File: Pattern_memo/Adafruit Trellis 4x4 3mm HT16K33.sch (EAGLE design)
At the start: 41 parts, among them U1 HT16K33 28SOP

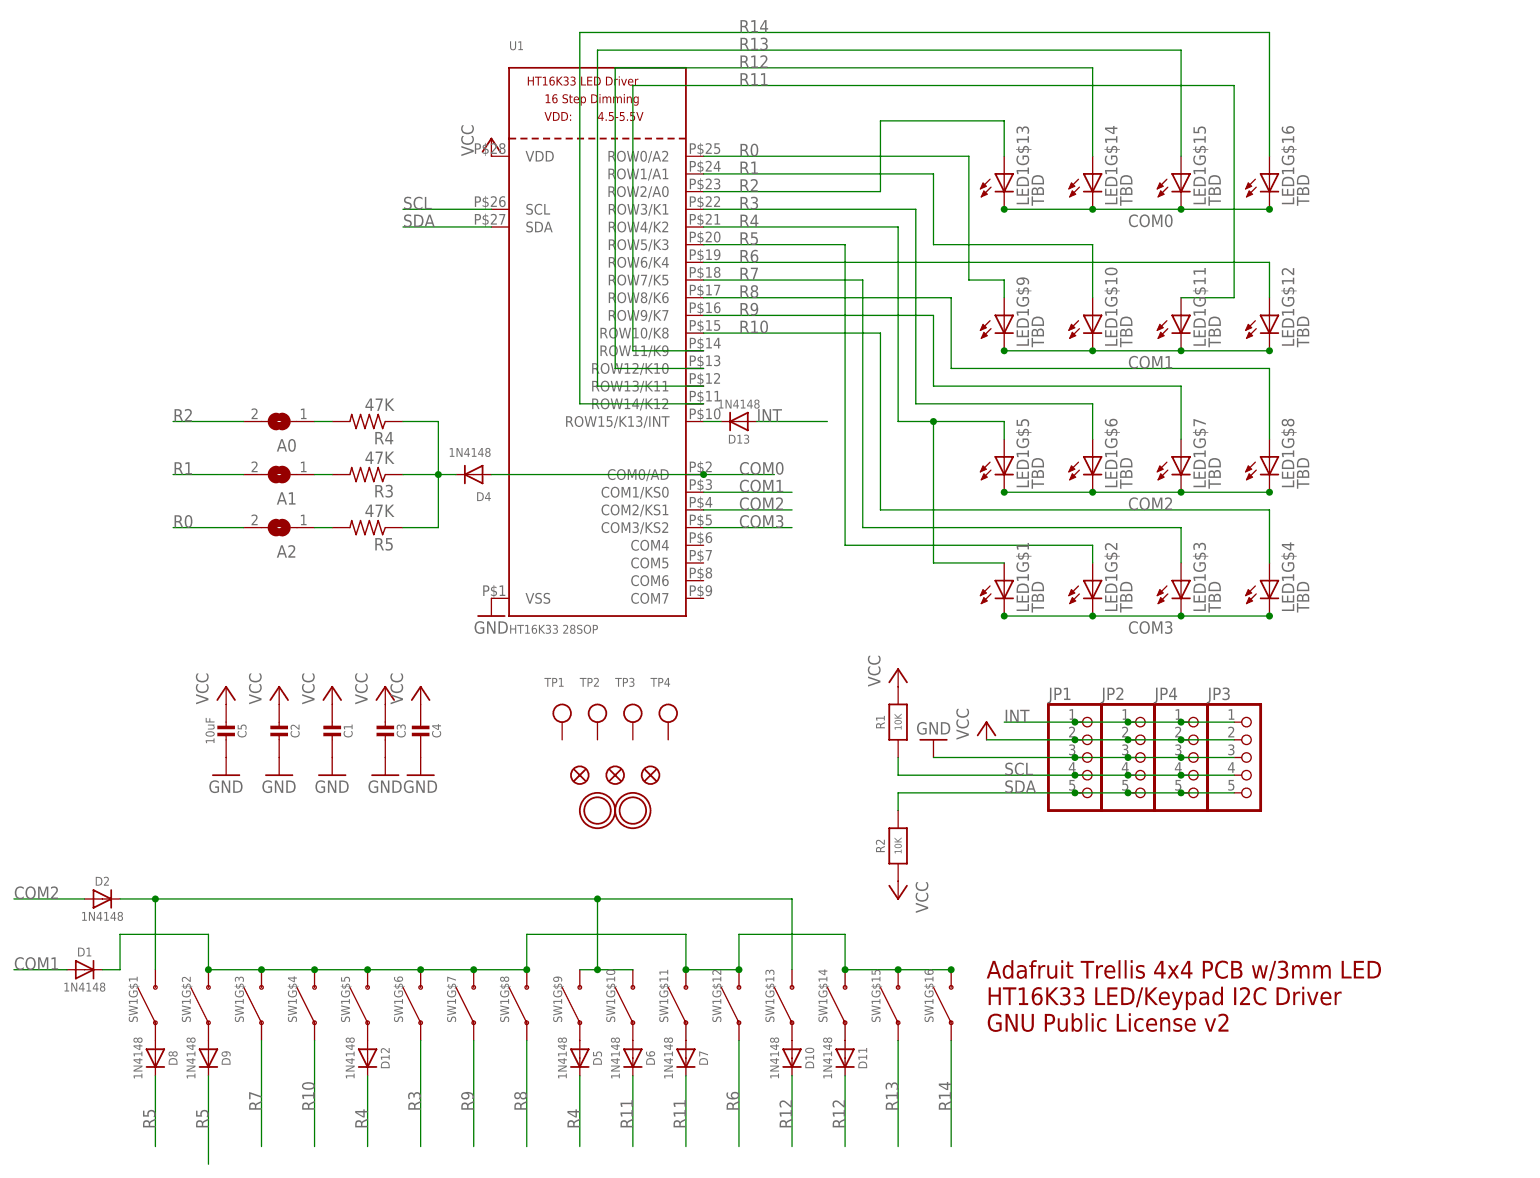
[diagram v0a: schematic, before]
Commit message: updated pcb board
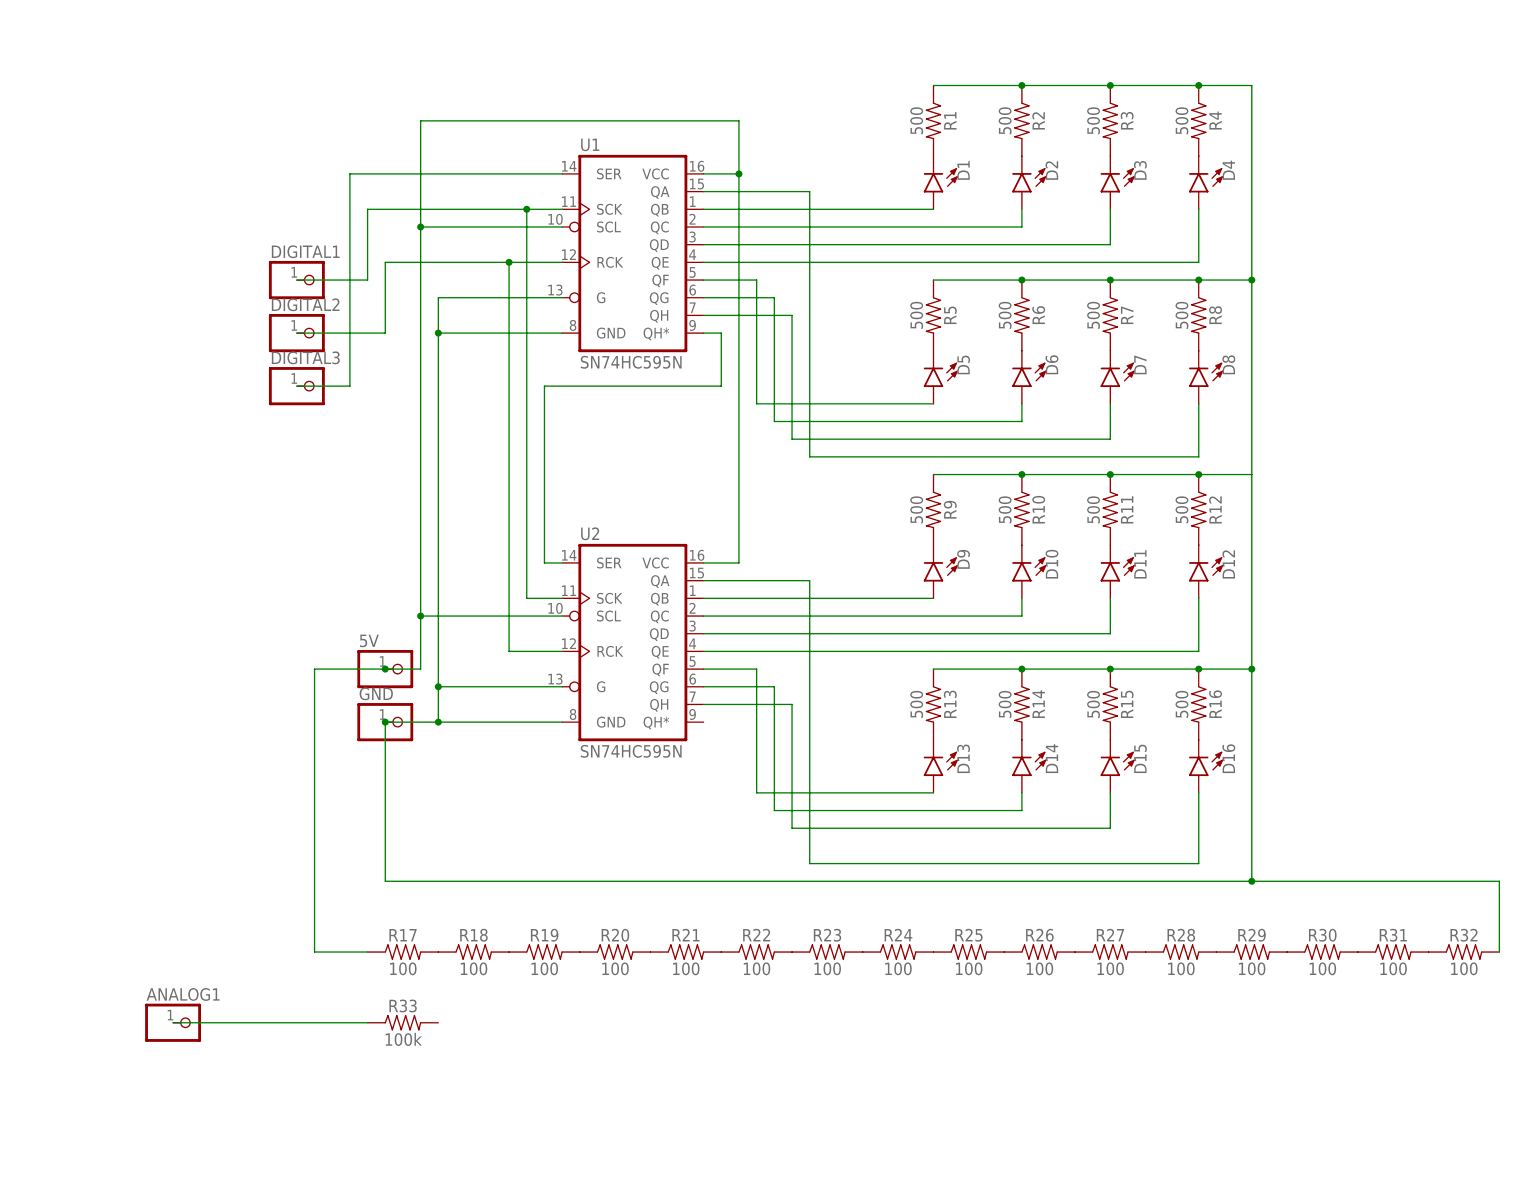
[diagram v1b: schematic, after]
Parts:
- removed A0, A1, A2: (no value), microbuilder:SOLDERJUMPERREFLOW_NOPASTE
- removed C1, C2, C3, C4: (no value), microbuilder:CAP_CERAMIC_0805
- removed C5: 10uF, microbuilder:CAP_CERAMIC_0805
- removed FID1, FID2, FID3: FIDUCIAL"", microbuilder:FIDUCIAL""
- removed JP1, JP2, JP3, JP4: (no value), microbuilder:HEADER-1X5EDGESMT
- removed LED1: TBD, microbuilder:LED-3MM-4X4GRID-3MM
- removed SW1: (no value), microbuilder:SWITCH-SILICON-4X4GRID-10MM-5.4MM
- removed TP1, TP2, TP3, TP4: (no value), microbuilder:TESTPOINT
- removed U$1, U$2: MOUNTINGHOLE2.5, microbuilder:MOUNTINGHOLE2.5
- added 5V, ANALOG1, DIGITAL1, DIGITAL2, DIGITAL3, GND: (no value), adafruit:PINHD-1X1
- added D14, D15, D16, D3: (no value), SparkFun-LED:LED3MM
- added R10, R11, R12, R13, R14, R15, R16, R6, R7, R8, R9: 500, SparkFun-Resistors:RESISTOR0603
- added R17, R18, R19, R20, R21, R22, R23, R24, R25, R26, R27, R28, R29, R30, R31, R32: 100, SparkFun-Resistors:100OHM-0603-1/10W-1%
- added R33: 100k, SparkFun-Resistors:100KOHM-0603-1/10W-1%
- added U2: SN74HC595N, SparkFun-IC-Logic:74HC595N
- D1, D10, D11, D12, D13, D2, D5, D6, D7, D8, D9: value 1N4148 -> (none); device microbuilder:DIODESOD-323 -> SparkFun-LED:LED3MM
- D4: value 1N4148 -> (none); device adafruit:DIODESOD-323F -> SparkFun-LED:LED3MM
- R1, R2: value 10K -> 500; device microbuilder:RESISTOR_0805 -> SparkFun-Resistors:RESISTOR0603
- R3, R4, R5: value 47K -> 500; device rcl:R-US_R0805 -> SparkFun-Resistors:RESISTOR0603
- U1: value HT16K33 28SOP -> SN74HC595N; device microbuilder:HT16K33_SOP28 -> SparkFun-IC-Logic:74HC595N
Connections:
- removed net COM0: D4.A, LED1G$13.C, LED1G$14.C, LED1G$15.C, LED1G$16.C, U1.COM0/AD
- removed net COM1: D1.A, LED1G$10.C, LED1G$11.C, LED1G$12.C, LED1G$9.C, U1.COM1/KS0
- removed net COM2: D2.A, LED1G$5.C, LED1G$6.C, LED1G$7.C, LED1G$8.C, U1.COM2/KS1
- removed net COM3: LED1G$1.C, LED1G$2.C, LED1G$3.C, LED1G$4.C, U1.COM3/KS2
- removed net GND: C1.1, C2.1, C3.1, C4.1, C5.1, JP1.3, JP2.3, JP3.3, JP4.3, U1.VSS
- removed net INT: D13.A, JP1.1, JP2.1, JP3.1, JP4.1
- removed net R0: A2.2, LED1G$9.A, U1.ROW0/A2
- removed net R1: A1.2, LED1G$10.A, U1.ROW1/A1
- removed net R10: LED1G$4.A, SW1G$4.P$1, U1.ROW10/K8
- removed net R11: D6.C, D7.C, LED1G$11.A, U1.ROW11/K9
- removed net R12: D10.C, D11.C, LED1G$14.A, U1.ROW12/K10
- removed net R13: LED1G$15.A, SW1G$15.P$1, U1.ROW13/K11
- removed net R14: LED1G$16.A, SW1G$16.P$1, U1.ROW14/K12
- removed net R2: A0.2, LED1G$13.A, U1.ROW2/A0
- removed net R3: LED1G$6.A, SW1G$6.P$1, U1.ROW3/K1
- removed net R4: D12.C, D5.C, LED1G$1.A, LED1G$5.A, U1.ROW4/K2
- removed net R5: D8.C, D9.C, LED1G$2.A, U1.ROW5/K3
- removed net R6: LED1G$12.A, SW1G$12.P$1, U1.ROW6/K4
- removed net R7: LED1G$3.A, SW1G$3.P$1, U1.ROW7/K5
- removed net R8: LED1G$8.A, SW1G$8.P$1, U1.ROW8/K6
- removed net R9: LED1G$7.A, SW1G$7.P$1, U1.ROW9/K7
- removed net SCL: JP1.4, JP2.4, JP3.4, JP4.4, R1.1, U1.SCL
- removed net SDA: JP1.5, JP2.5, JP3.5, JP4.5, R2.2, U1.SDA
- removed net VCC: C1.2, C2.2, C3.2, C4.2, C5.2, JP1.2, JP2.2, JP3.2, JP4.2, R1.2, R2.1, U1.VDD
- new net N$13: D7.C, R7.2
- new net N$14: GND.1, R1.1, R10.1, R11.1, R12.1, R13.1, R14.1, R15.1, R16.1, R2.1, R3.1, R32.2, R4.1, R5.1, R6.1, R7.1, R8.1, R9.1, U1.G, U1.GND, U2.G, U2.GND
- new net N$15: D8.C, R8.2
- new net N$17: D10.C, R10.2
- new net N$18: D11.C, R11.2
- new net N$21: D14.C, R14.2
- new net N$22: D15.C, R15.2
- new net N$23: D16.C, R16.2
- new net N$24: D1.A, U1.QB
- new net N$25: D2.A, U1.QC
- new net N$26: D3.A, U1.QD
- new net N$27: D4.A, U1.QE
- new net N$28: D5.A, U1.QF
- new net N$29: D6.A, U1.QG
- new net N$30: D7.A, U1.QH
- new net N$31: D8.A, U1.QA
- new net N$32: D9.A, U2.QB
- new net N$33: D10.A, U2.QC
- new net N$34: D11.A, U2.QD
- new net N$35: 5V.1, R17.1, U1.SCL, U1.VCC, U2.SCL, U2.VCC
- new net N$36: D12.A, U2.QE
- new net N$37: R18.2, R19.1
- new net N$38: D13.A, U2.QF
- new net N$39: D14.A, U2.QG
- new net N$40: R19.2, R20.1
- new net N$41: D15.A, U2.QH
- new net N$42: R20.2, R21.1
- new net N$43: R21.2, R22.1
- new net N$44: R22.2, R23.1
- new net N$45: R23.2, R24.1
- new net N$46: R24.2, R25.1
- new net N$47: R25.2, R26.1
- new net N$48: R26.2, R27.1
- new net N$49: R27.2, R28.1
- new net N$50: R28.2, R29.1
- new net N$51: R29.2, R30.1
- new net N$52: R30.2, R31.1
- new net N$53: R31.2, R32.1
- new net N$54: D16.A, U2.QA
- net N$1: now also R17.2, R18.1; no longer D2.C, SW1G$1.P$2, SW1G$10.P$2, SW1G$13.P$2, SW1G$9.P$2
- net N$10: now also D4.C, R4.2; no longer D10.A, SW1G$13.P$1
- net N$11: now also D5.C, R5.2; no longer D11.A, SW1G$14.P$1
- net N$12: now also D6.C, R6.2; no longer D12.A, SW1G$5.P$1
- net N$16: now also D9.C, R9.2; no longer D4.C, R3.1, R4.1, R5.1
- net N$19: now also D12.C, R12.2; no longer A1.1, R3.2
- net N$2: now also ANALOG1.1, R33.1; no longer D13.C, U1.ROW15/K13/INT
- net N$20: now also D13.C, R13.2; no longer A0.1, R4.2
- net N$3: now also DIGITAL3.1, U1.SER; no longer D5.A, SW1G$9.P$1
- net N$4: now also DIGITAL1.1, U1.SCK, U2.SCK; no longer D6.A, SW1G$10.P$1
- net N$5: now also DIGITAL2.1, U1.RCK, U2.RCK; no longer D1.C, SW1G$11.P$2, SW1G$12.P$2, SW1G$14.P$2, SW1G$15.P$2, SW1G$16.P$2, SW1G$2.P$2, SW1G$3.P$2, SW1G$4.P$2, SW1G$5.P$2, SW1G$6.P$2, SW1G$7.P$2, SW1G$8.P$2
- net N$6: now also D1.C, R1.2; no longer D7.A, SW1G$11.P$1
- net N$7: now also D2.C, R2.2; no longer D8.A, SW1G$1.P$1
- net N$8: now also U1.QH*, U2.SER; no longer D9.A, SW1G$2.P$1
- net N$9: now also D3.C, R3.2; no longer A2.1, R5.2
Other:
- note removed: "Adafruit Trellis 4x4 PCB w/3mm LED HT16K33 LED/Keypad I2C Driver GNU Public License v2"
- moved on the sheet: R3, R4, R5

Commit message: schematic & board finished
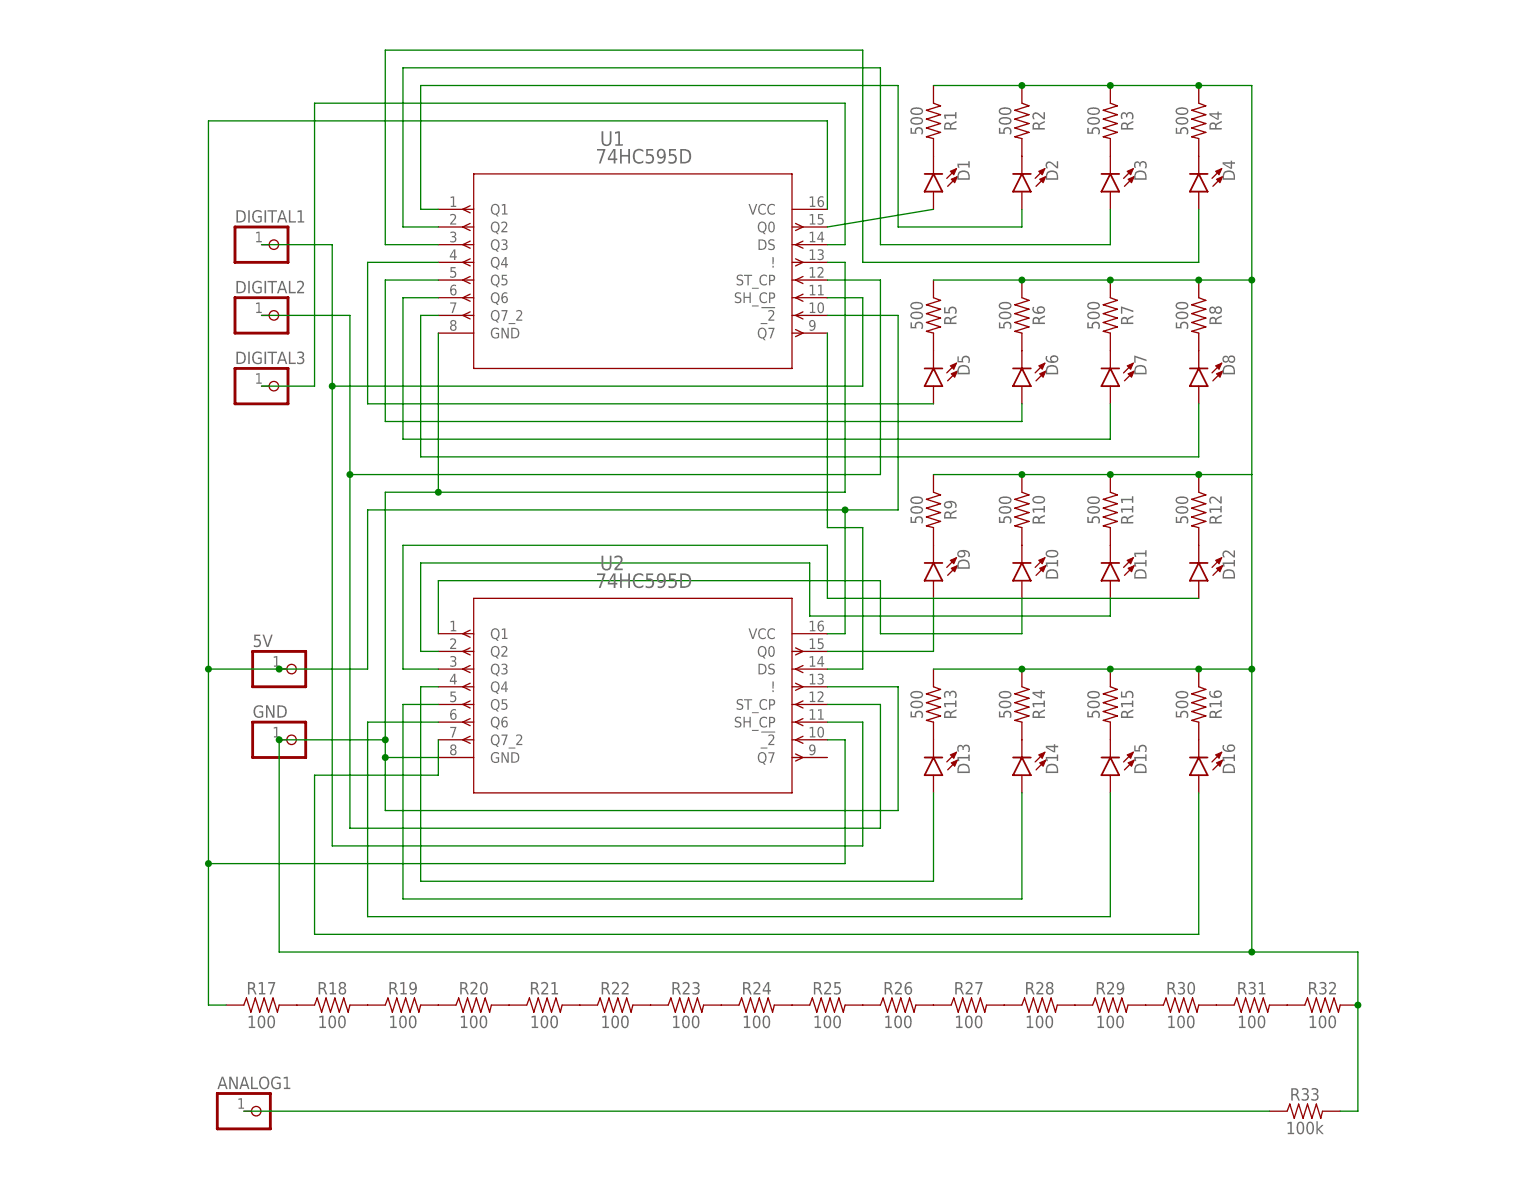
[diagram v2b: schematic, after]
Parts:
- U1, U2: value SN74HC595N -> 74HC595D; device SparkFun-IC-Logic:74HC595N -> Shift_Register:74HC595D
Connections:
- removed net N$34: D11.A, U2.QD
- new net N$55: DIGITAL1.1, U1.SH_CP, U2.SH_CP
- net N$14: now also D1.A, U1.Q0; no longer GND.1, R1.1, R10.1, R11.1, R12.1, R13.1, R14.1, R15.1, R16.1, R2.1, R3.1, R32.2, R4.1, R5.1, R6.1, R7.1, R8.1, R9.1, U1.G, U1.GND, U2.G, U2.GND
- net N$24: now also D5.A, U1.Q4; no longer D1.A, U1.QB
- net N$25: now also U1.Q1; no longer U1.QC
- net N$26: now also U1.Q2; no longer U1.QD
- net N$27: now also U1.Q3; no longer U1.QE
- net N$28: now also U1.Q7, U2.DS; no longer D5.A, U1.QF
- net N$29: now also U1.Q5; no longer U1.QG
- net N$3: now also U1.DS; no longer U1.SER
- net N$30: now also U1.Q6; no longer U1.QH
- net N$31: now also U1.Q7_2; no longer U1.QA
- net N$32: now also D13.A, U2.Q4; no longer D9.A, U2.QB
- net N$33: now also U2.Q1; no longer U2.QC
- net N$35: now also U1.!_2, U2.!_2; no longer U1.SCL, U2.SCL
- net N$36: now also U2.Q3; no longer U2.QE
- net N$38: now also D9.A, U2.Q0; no longer D13.A, U2.QF
- net N$39: now also U2.Q5; no longer U2.QG
- net N$4: now also D11.A, U2.Q2; no longer DIGITAL1.1, U1.SCK, U2.SCK
- net N$41: now also U2.Q6; no longer U2.QH
- net N$5: now also U1.ST_CP, U2.ST_CP; no longer U1.RCK, U2.RCK
- net N$54: now also U2.Q7_2; no longer U2.QA
- net N$8: now also GND.1, R1.1, R10.1, R11.1, R12.1, R13.1, R14.1, R15.1, R16.1, R2.1, R3.1, R32.2, R33.2, R4.1, R5.1, R6.1, R7.1, R8.1, R9.1, U1.!, U1.GND, U2.!, U2.GND; no longer U1.QH*, U2.SER
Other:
- moved on the sheet: 5V, ANALOG1, DIGITAL1, DIGITAL2, DIGITAL3, GND, R17, R18, R19, R20, R21, R22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
